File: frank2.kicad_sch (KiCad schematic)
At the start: 4 parts, among them J1 USB Data, J2 Keyboard Data

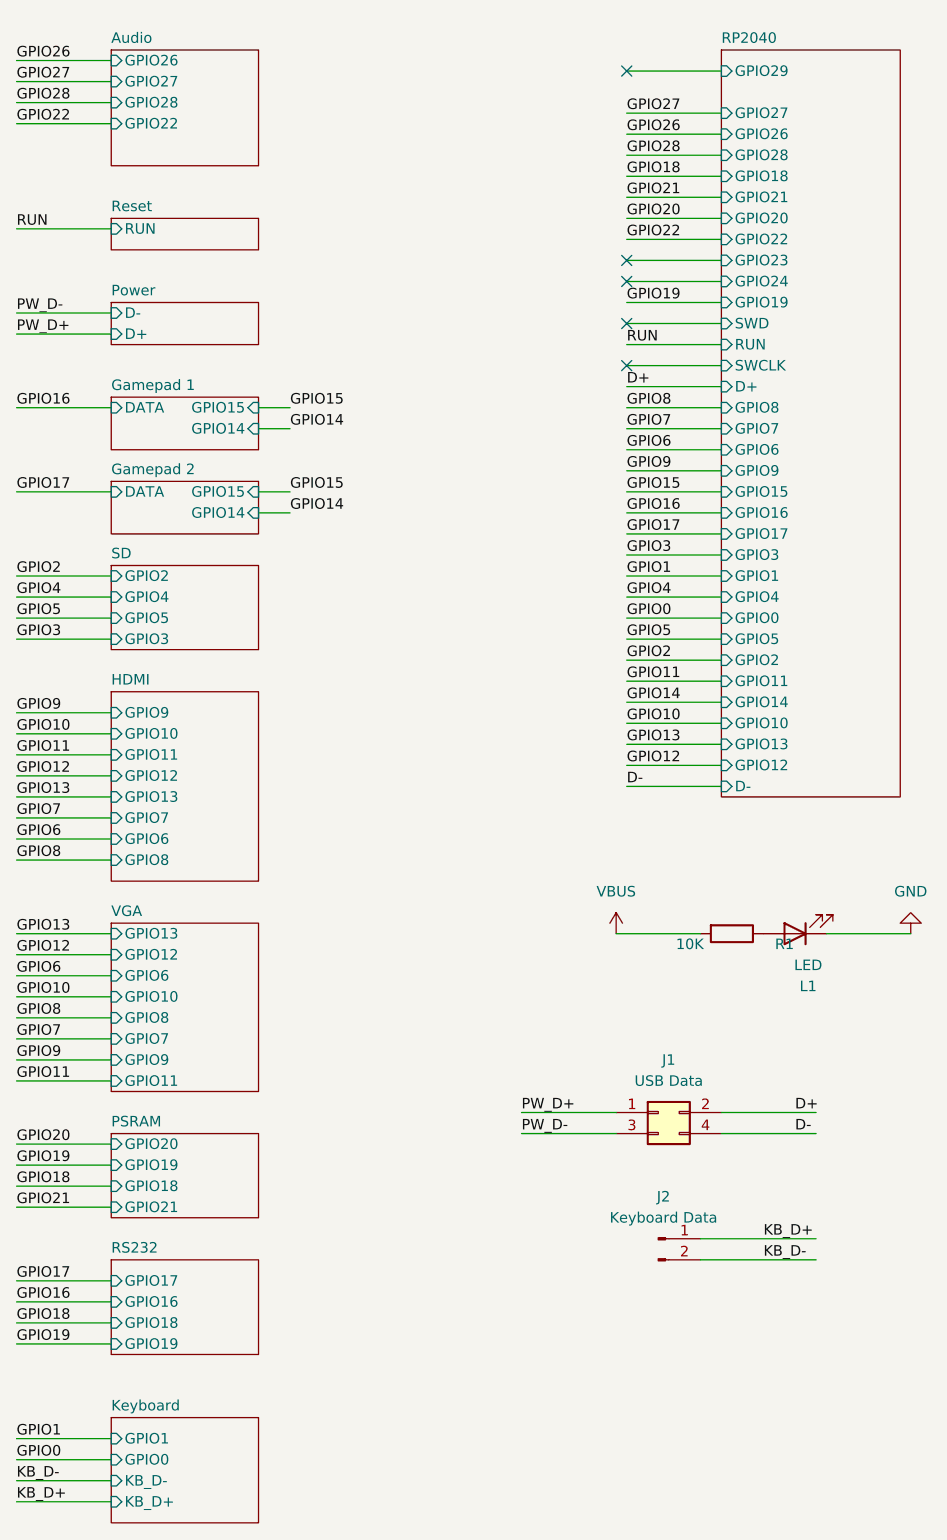
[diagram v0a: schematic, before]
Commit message: HW Rev 1.0
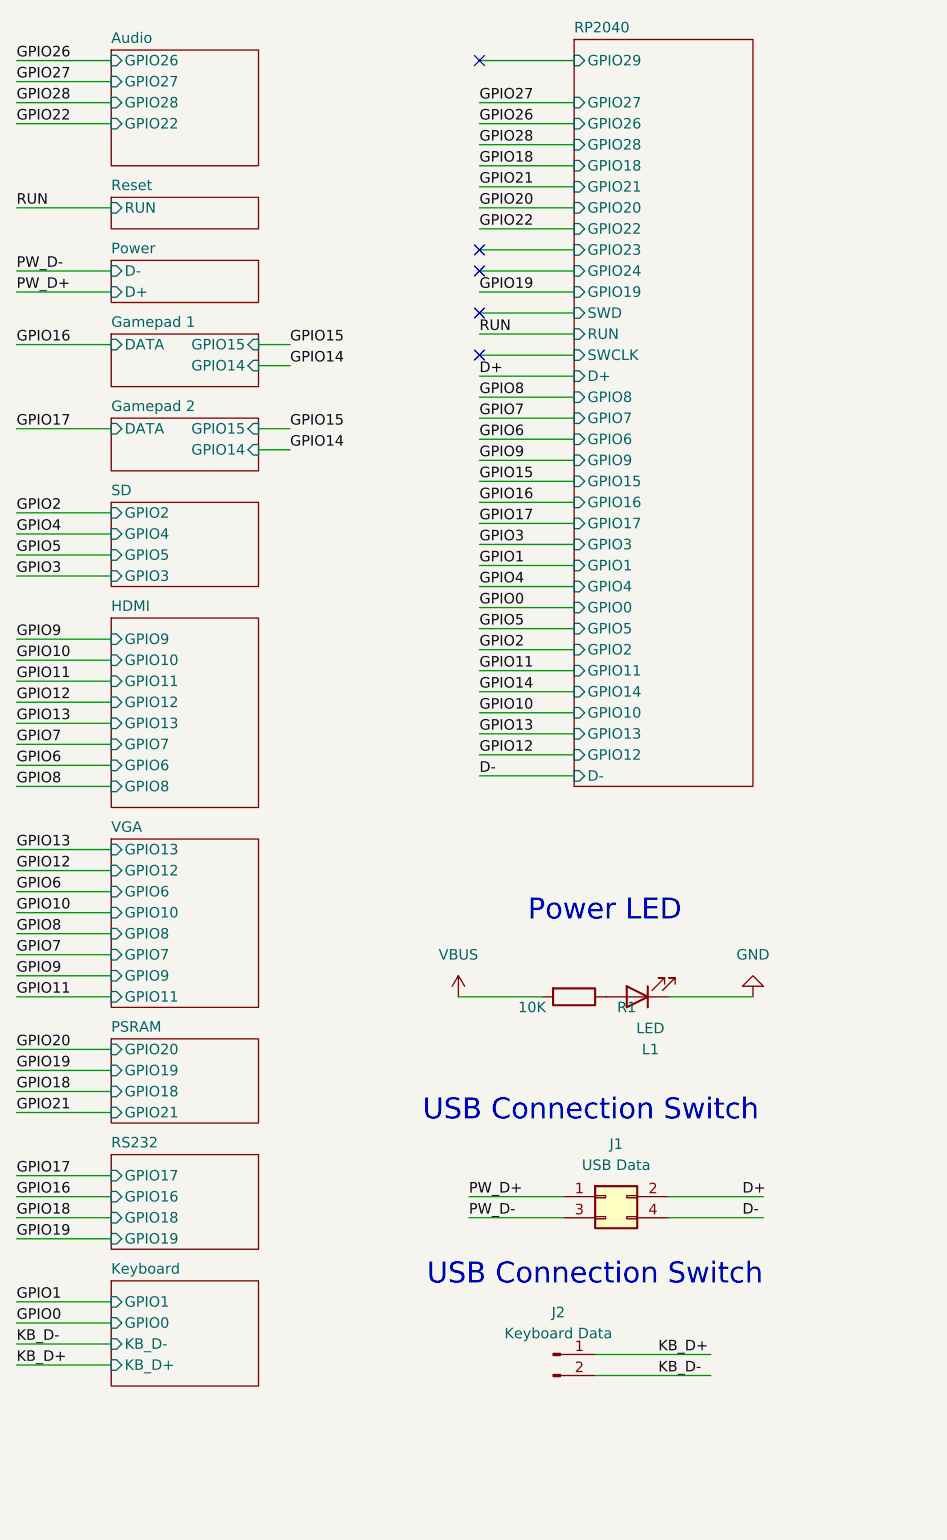
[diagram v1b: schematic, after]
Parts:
- J1: footprint Connector_PinHeader_2.54mm:PinHeader_2x02_P2.54mm_Vertical -> LIBS:Medved_2x02
- J2: footprint Connector_PinHeader_2.54mm:PinHeader_1x02_P2.54mm_Vertical -> LIBS:Medved_PinHeader_1x02
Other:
- note added: "Power LED"
- note added: "USB Connection Switch"
- moved on the sheet: J1, J2, L1, R1
